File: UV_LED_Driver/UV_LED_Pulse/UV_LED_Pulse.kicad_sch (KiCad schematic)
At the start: 25 parts, among them J1 PWR/Signal, Q1 BC817, Q2 2N7002

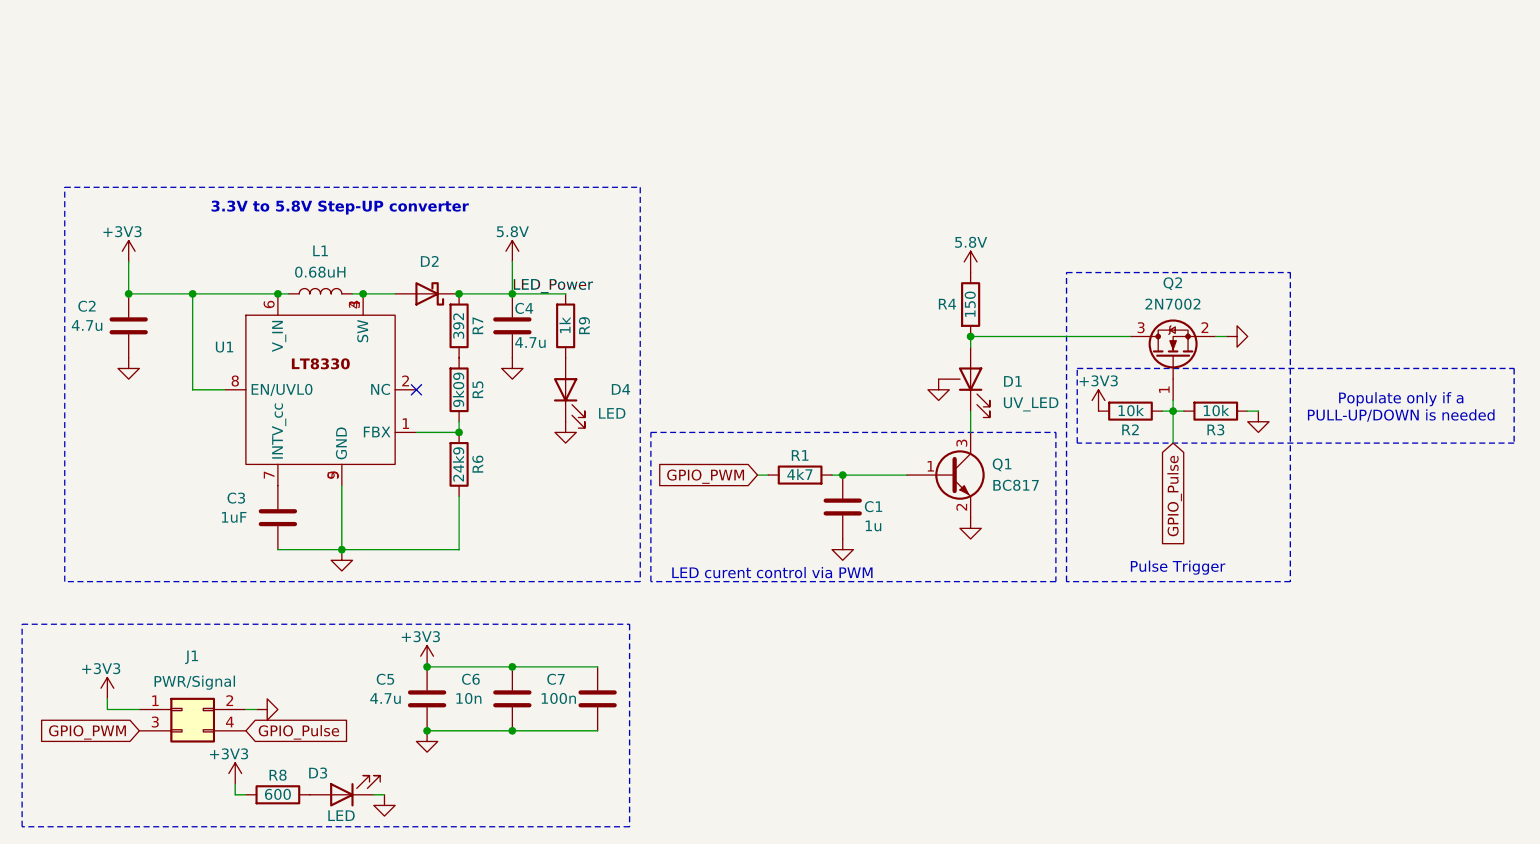
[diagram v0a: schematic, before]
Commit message: .
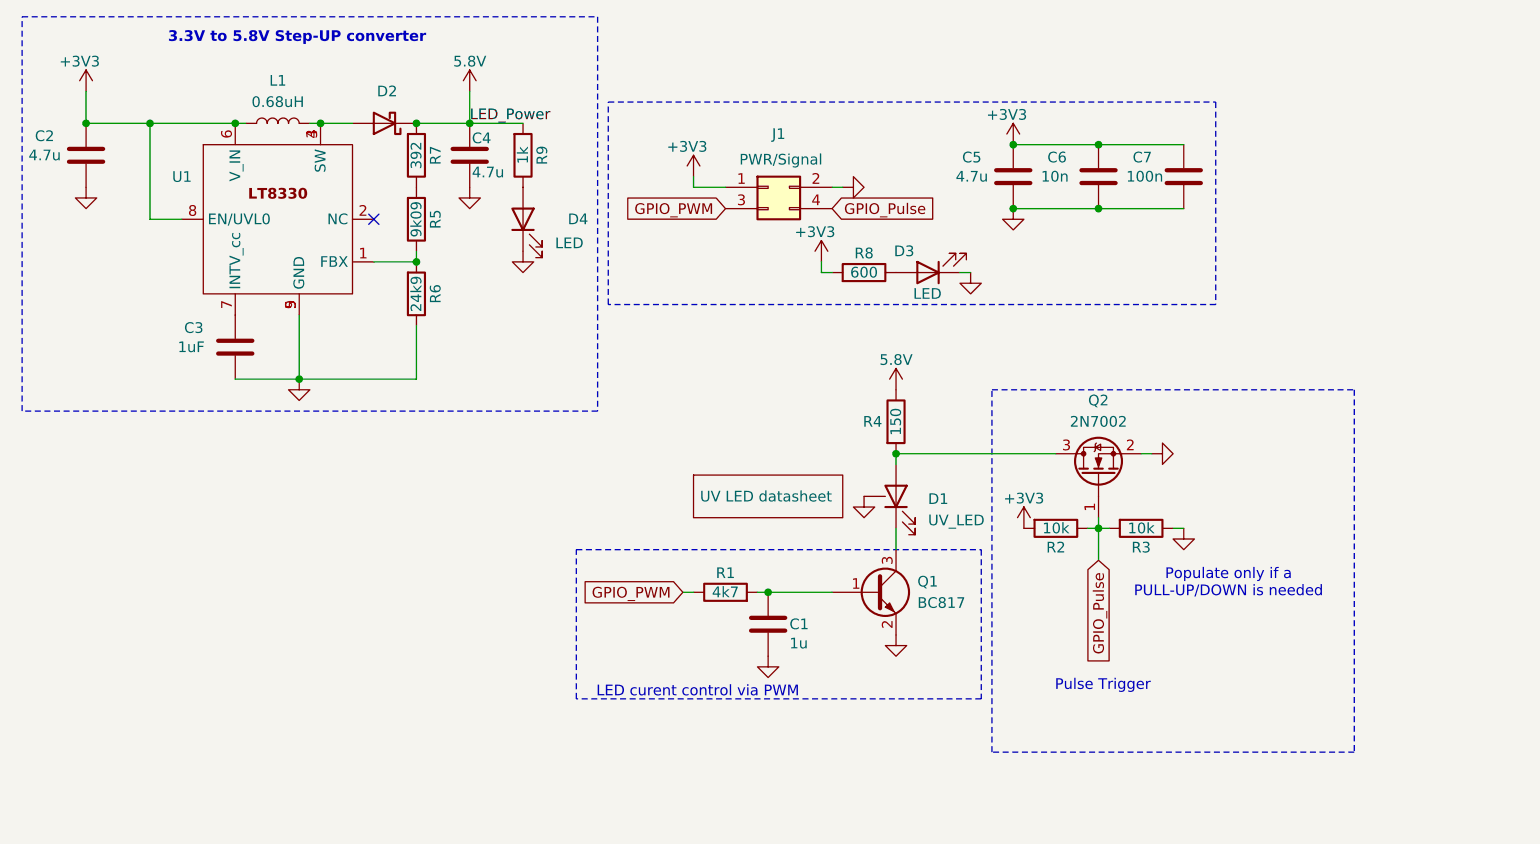
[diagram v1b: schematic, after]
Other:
- added sheet UV LED datasheet (Wavelength_Intensity.kicad_sch)
- moved on the sheet: C1, C2, C3, C4, C5, C6, C7, D1, D2, D3, D4, J1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
